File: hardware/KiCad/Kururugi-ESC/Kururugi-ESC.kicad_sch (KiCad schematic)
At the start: 78 parts, among them J1 Conn_01x01, J2 Conn_01x01, J3 Conn_01x01, J4 Conn_01x01, J5 Conn_01x01, J6 Conn_01x01, J7 Conn_01x01, J8 JTAG_TC2030, U1 STM32G484CEU6, U2 LM5160A, U3 TPS7B92033, X1 16MHz

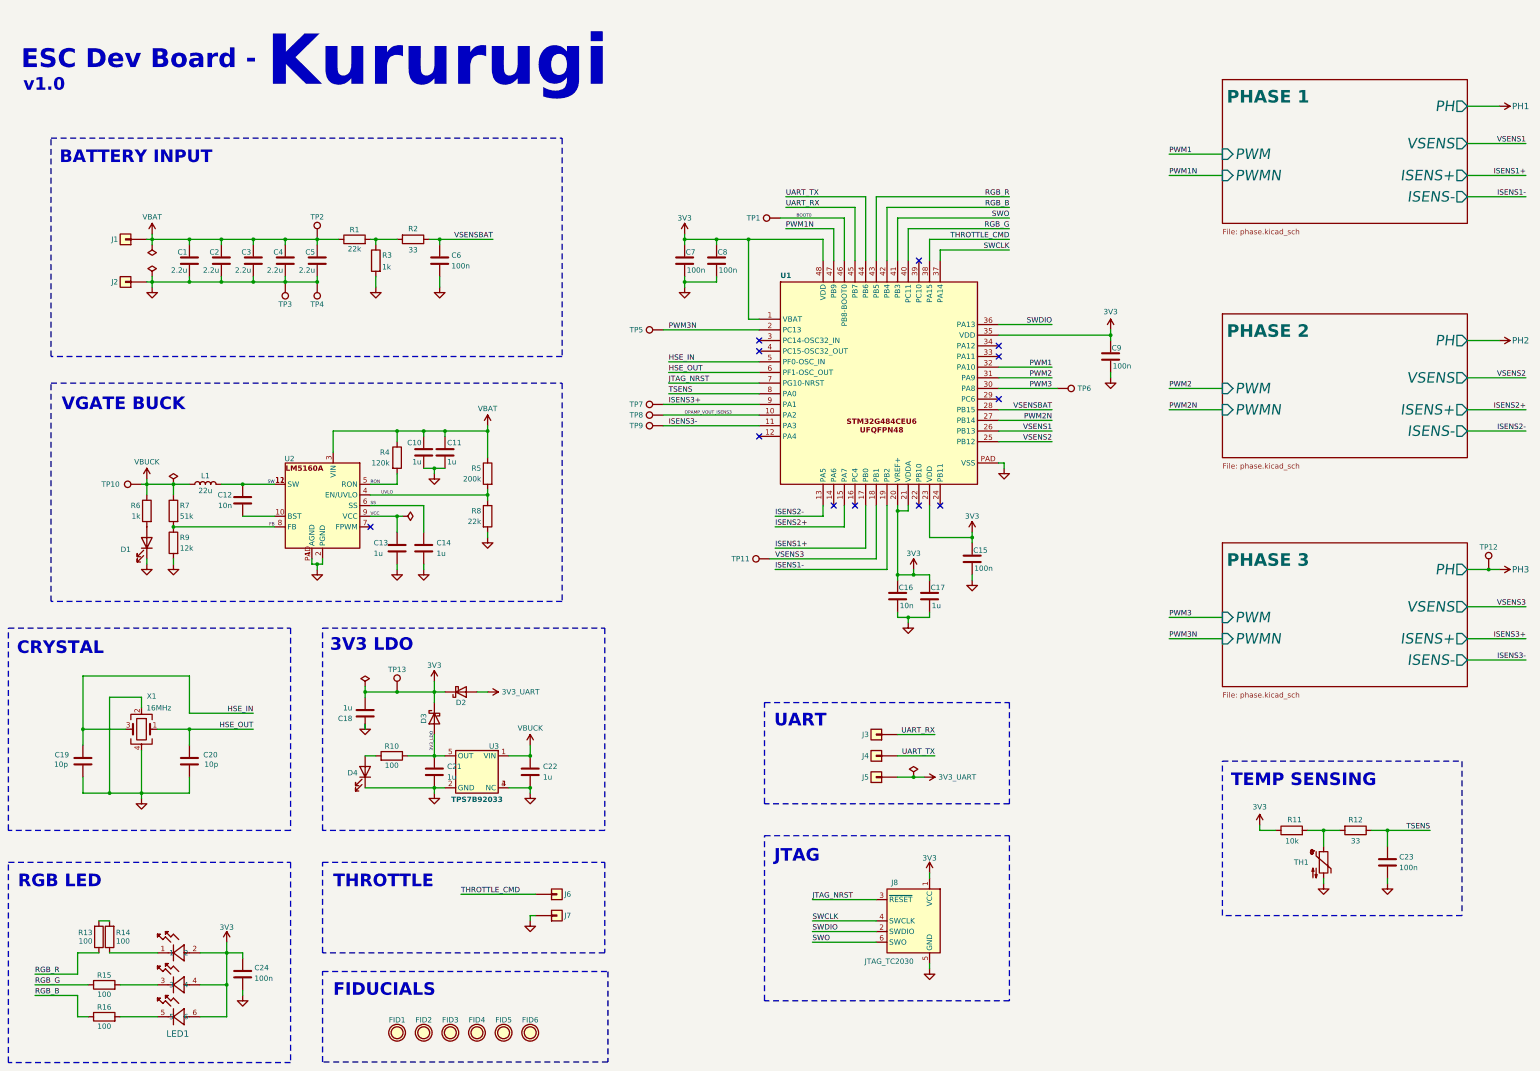
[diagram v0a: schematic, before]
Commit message: Kicad minor corrections
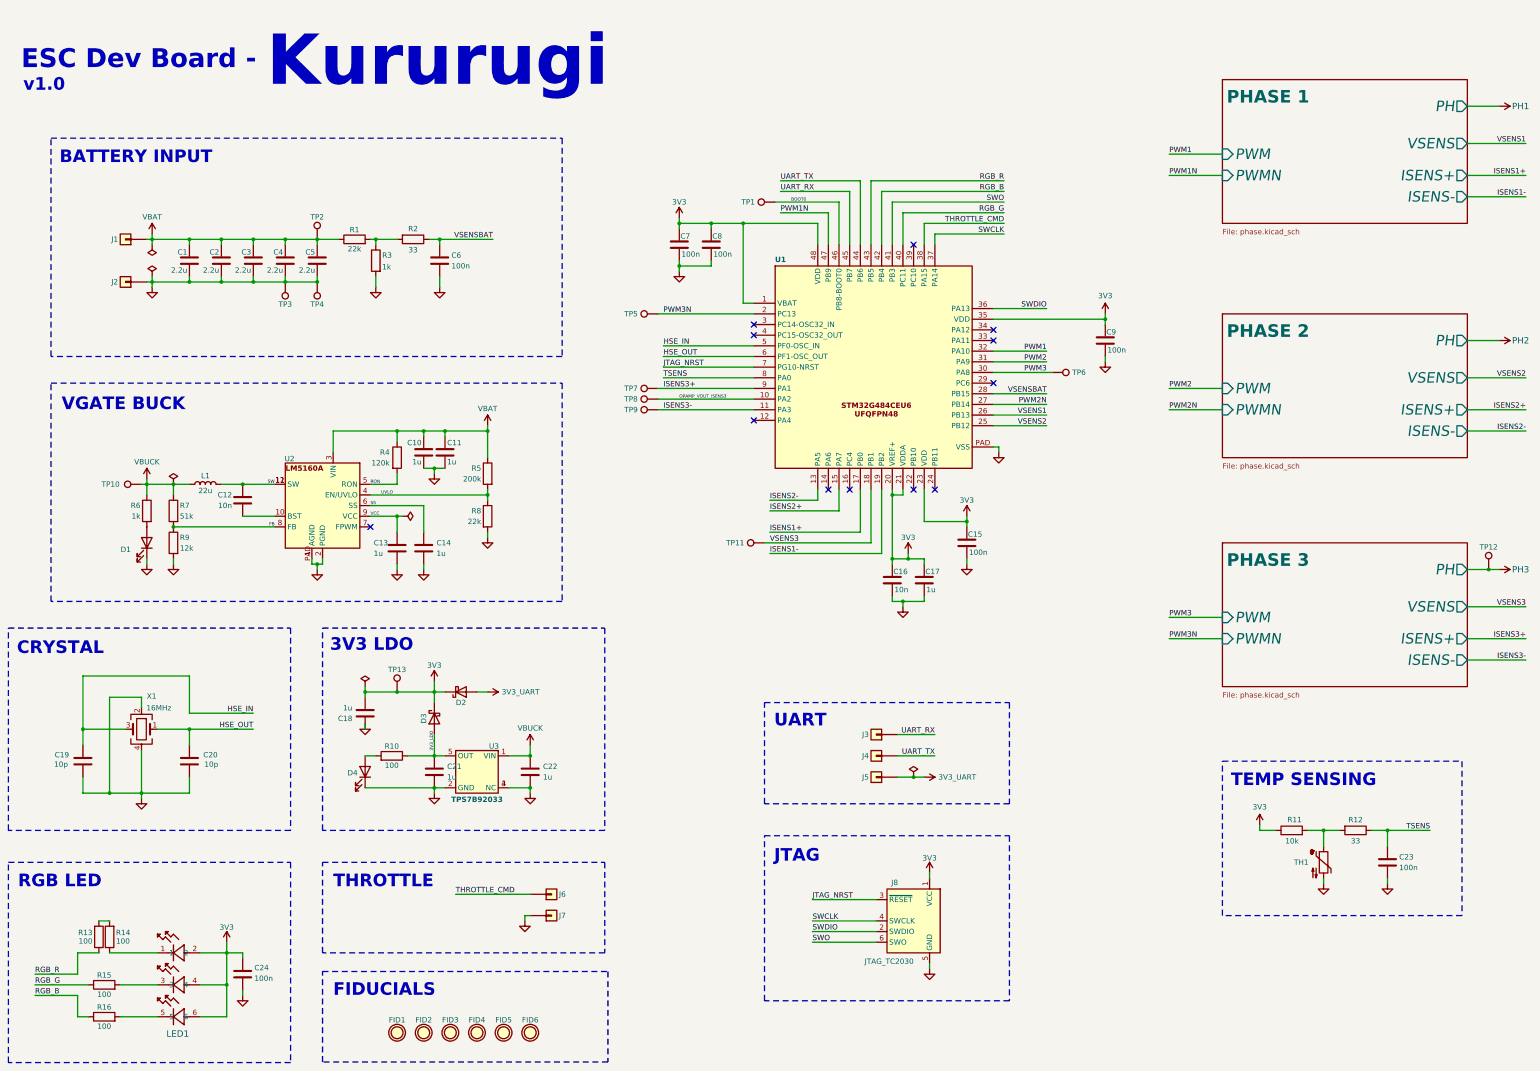
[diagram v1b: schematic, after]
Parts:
- R12, R2: LCSC C25752 -> C25105
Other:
- moved on the sheet: C15, C16, C17, C7, C8, C9, J6, J7, TP1, TP11, TP5, TP6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
